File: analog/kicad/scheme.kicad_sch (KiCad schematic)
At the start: 17 parts, among them U1 LM324

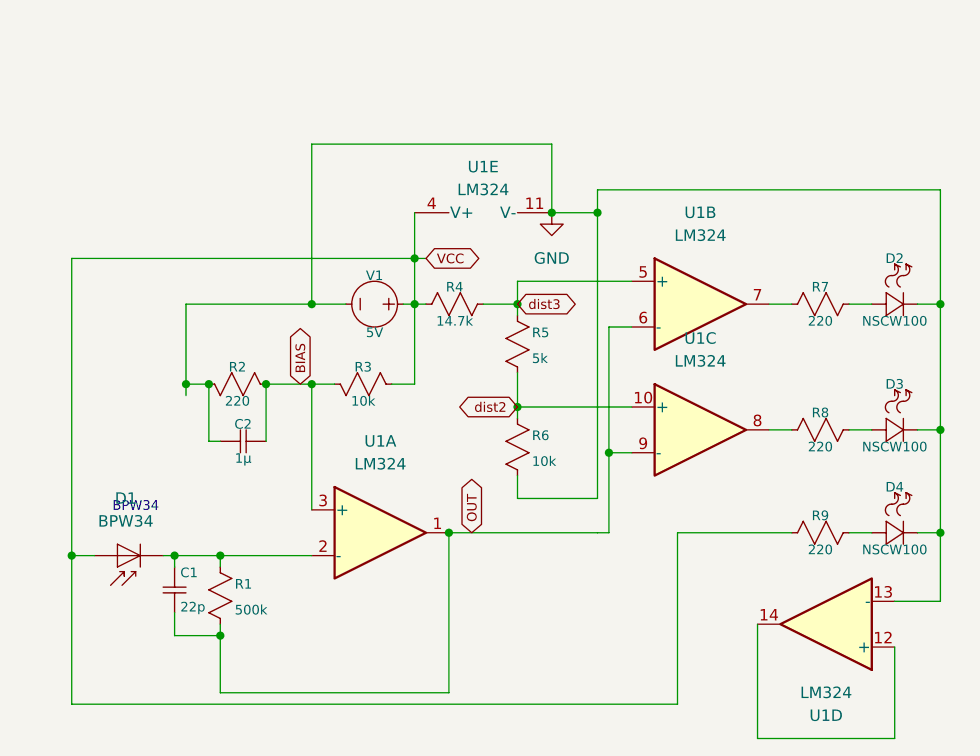
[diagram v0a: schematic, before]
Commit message: restructuring analog
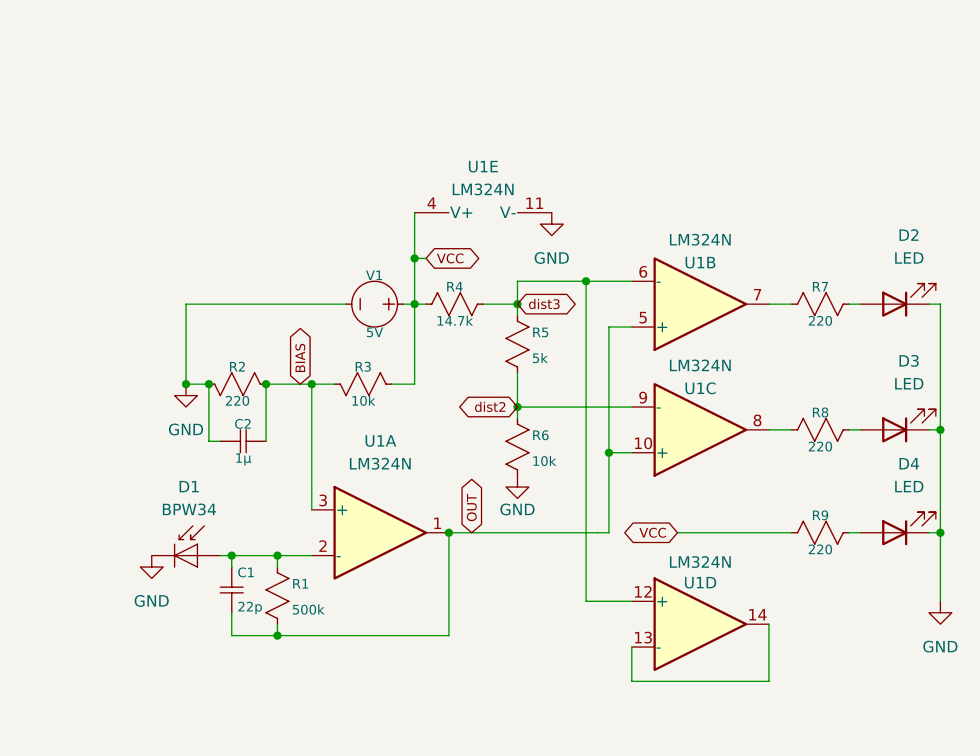
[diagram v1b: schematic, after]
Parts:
- removed D2, D3, D4: NSCW100, symbol ltspice:LED
- added D2, D3, D4: LED, symbol Device:LED
- U1: value LM324 -> LM324N; footprint (none) -> Package_DIP:DIP-14_W7.62mm
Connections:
- net GND: now also D1.1 (K), D2.1 (K), D3.1 (K), D4.1 (K); no longer U1.13 (-)
- net OUT: now also U1.10 (+), U1.5 (+); no longer U1.6 (-), U1.9 (-)
- net VCC: no longer D1.2 (A)
- net dist2: now also U1.9 (-); no longer U1.10 (+)
- net dist3: now also U1.12 (+), U1.6 (-); no longer U1.5 (+)
- net at C1.1, R1.1, U1.2 (-): now also D1.2 (A); no longer D1.1 (K)
- net at R8.1: now also D3.2 (A)
- net at R7.1: now also D2.2 (A)
- net at R9.1: now also D4.2 (A)
- net at U1.14: now also U1.13 (-); no longer U1.12 (+)
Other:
- note removed: "BPW34"
- moved on the sheet: C1, R1

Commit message: kicad pcb and other fixes
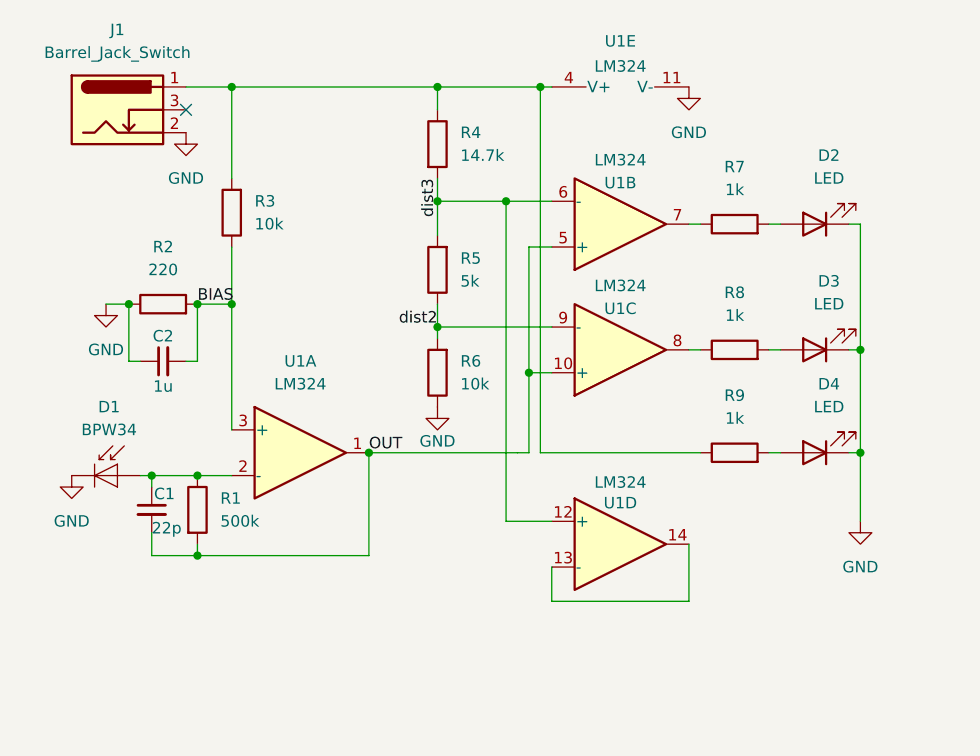
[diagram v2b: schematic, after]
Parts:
- removed C1: 22p, symbol ltspice:cap
- removed C2: 1µ, symbol ltspice:cap
- removed R1: 500k, symbol ltspice:res
- removed R2, R7, R8, R9: 220, symbol ltspice:res
- removed R3, R6: 10k, symbol ltspice:res
- removed R4: 14.7k, symbol ltspice:res
- removed R5: 5k, symbol ltspice:res
- removed V1: 5V, symbol ltspice:voltage
- added C1: 22p, Capacitor_SMD:C_0603_1608Metric, symbol Device:C_Small
- added C2: 1u, Capacitor_SMD:C_0603_1608Metric, symbol Device:C_Small
- added J1: Barrel_Jack_Switch, Connector_BarrelJack:BarrelJack_GCT_DCJ200-10-A_Horizontal, symbol Connector:Barrel_Jack_Switch
- added R1: 500k, Resistor_SMD:R_0603_1608Metric, symbol Device:R
- added R2: 220, Resistor_SMD:R_0603_1608Metric, symbol Device:R
- added R3, R6: 10k, Resistor_SMD:R_0603_1608Metric, symbol Device:R
- added R4: 14.7k, Resistor_SMD:R_0603_1608Metric, symbol Device:R
- added R5: 5k, Resistor_SMD:R_0603_1608Metric, symbol Device:R
- added R7, R8, R9: 1k, Resistor_SMD:R_0603_1608Metric, symbol Device:R
- D2, D3, D4: footprint (none) -> LED_THT:LED_D5.0mm
- U1: value LM324N -> LM324; footprint Package_DIP:DIP-14_W7.62mm -> Package_DIP:DIP-14_W7.62mm_Socket
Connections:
- net BIAS: now also C2.2, R2.2, R3.1
- net GND: now also C2.1, J1.2, R2.1, R6.1
- net OUT: now also C1.2, R1.2
- net dist2: now also R5.1, R6.2
- net dist3: now also R4.2, R5.2
- net at D1.2 (A), U1.2 (-): now also C1.1, R1.1
- net at D3.2 (A): now also R8.2
- net at U1.8: now also R8.1
- net at D4.2 (A): now also R9.2
- net at D2.2 (A): now also R7.2
- net at U1.7: now also R7.1
- net VCC: no longer names the net of U1.4 (V+)
- net VCC: now also J1.1, R3.2, R4.1, R9.1
- no-connect marks 0 -> 1
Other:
- moved on the sheet: D1, D2, D3, D4, U1A, U1B, U1C, U1D, U1E
